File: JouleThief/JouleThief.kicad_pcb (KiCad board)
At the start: 2 copper layers, 55.3 x 13.2 mm, 11 parts, among them J1 Screw_Terminal_01x02, J2 Screw_Terminal_01x02, Q1 BC547, Q2 BC547

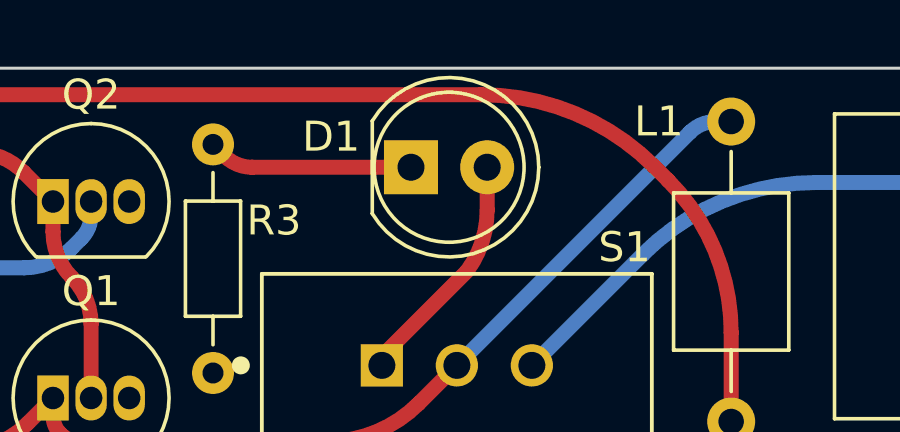
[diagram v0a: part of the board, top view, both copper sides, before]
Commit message: enh silkscreen
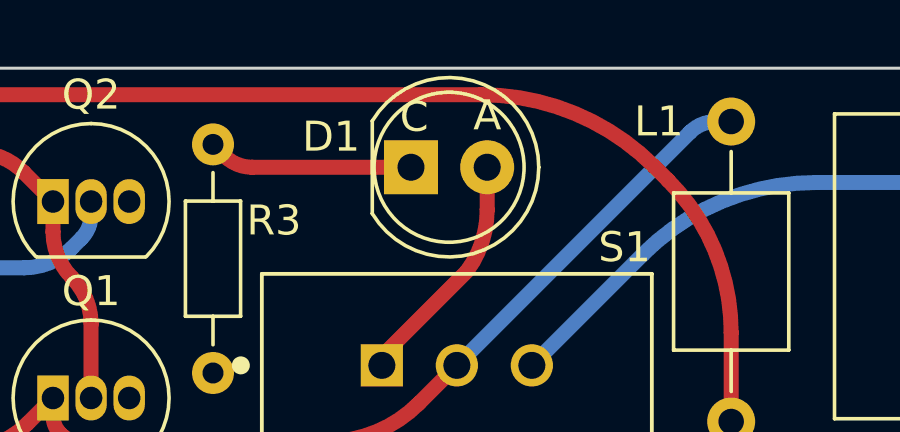
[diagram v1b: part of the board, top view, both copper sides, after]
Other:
- board text added: "A"
- board text added: "C"
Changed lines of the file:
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@@
     (effects (font (size 1 1) (thickness 0.25)) (justify mirror))
+  )
+  (gr_text "A" (at 153.924 93.5228) (layer "F.SilkS")
+    (effects (font (size 1 1) (thickness 0.25)))
+  )
+  (gr_text "C" (at 151.4856 93.5736) (layer "F.SilkS")
+    (effects (font (size 1 1) (thickness 0.25)))
   )
   (segment (start 130.93163 104.648) (end 136.533334 104.648) (width 0.5) (layer "F.Cu") (net 1))
